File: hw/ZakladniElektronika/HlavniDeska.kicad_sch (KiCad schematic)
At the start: 1 part

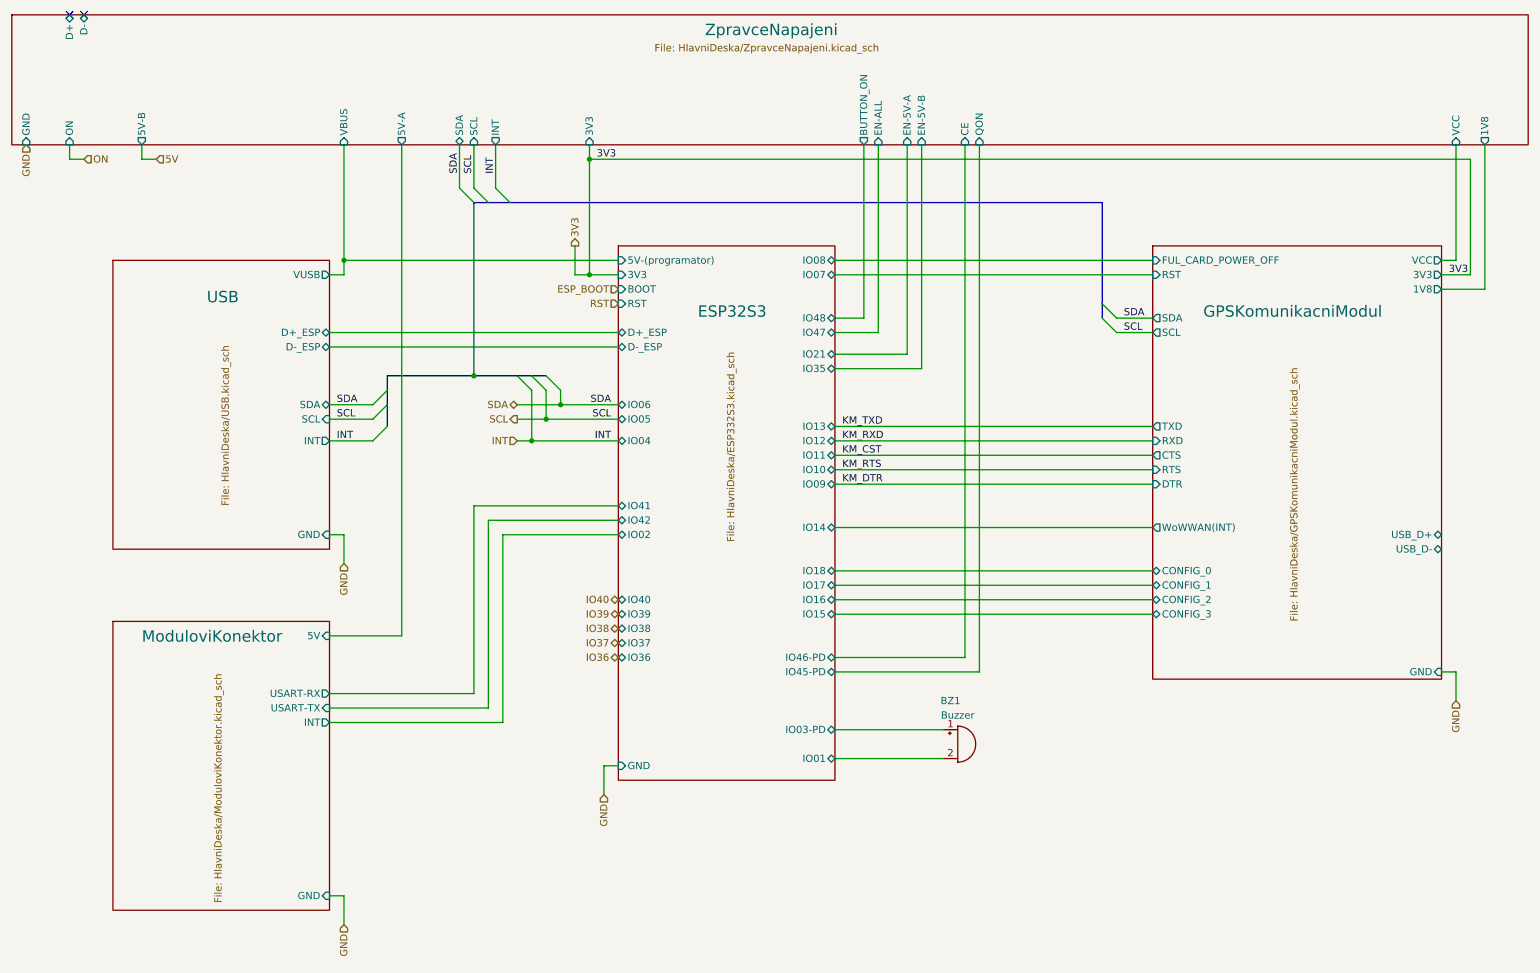
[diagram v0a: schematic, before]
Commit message: WIP
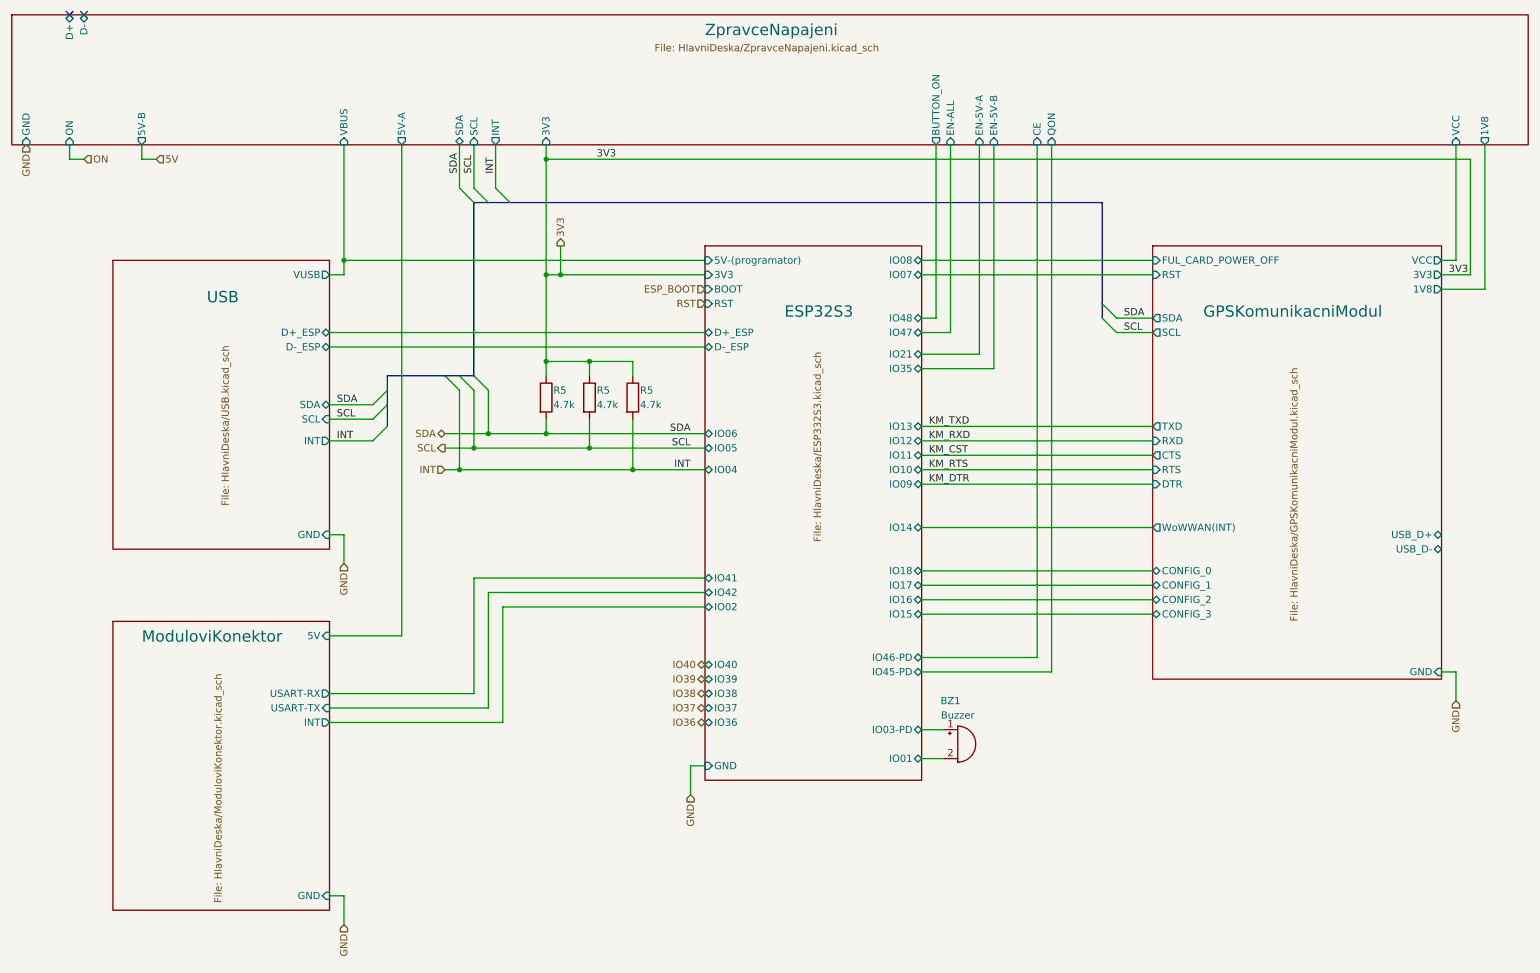
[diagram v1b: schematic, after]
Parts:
- added R5 (x3): 4.7k, Resistor_SMD:R_0201_0603Metric, symbol Device:R
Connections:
- net 3V3: now also R5.1, R5.1, R5.1
- net INT: now also R5.2
- net SCL: now also R5.2
- net SDA: now also R5.2
